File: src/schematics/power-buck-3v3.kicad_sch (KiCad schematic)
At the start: 12 parts, among them U14 INA219xxDCN, U4 TPS562202DRLR

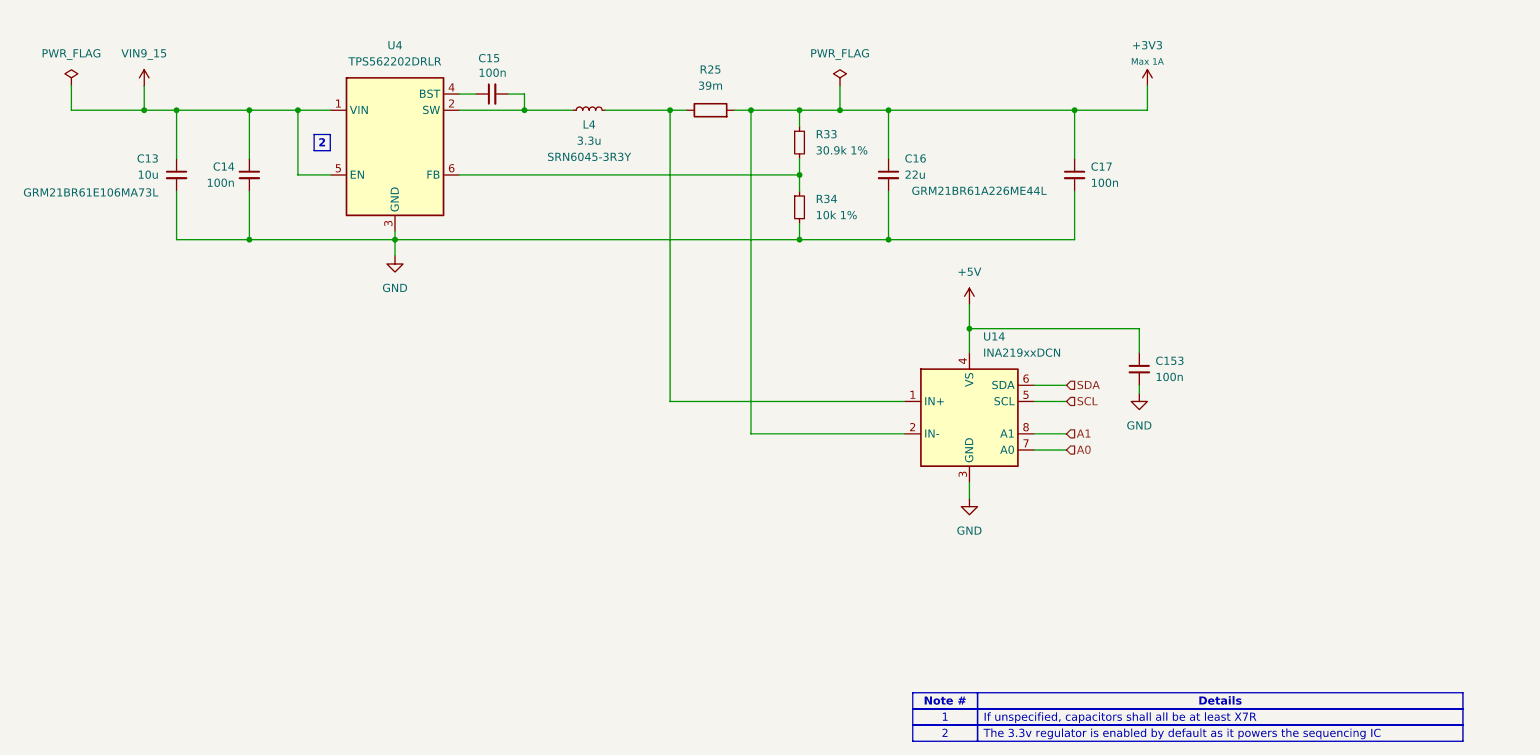
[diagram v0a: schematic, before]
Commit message: Add bom components
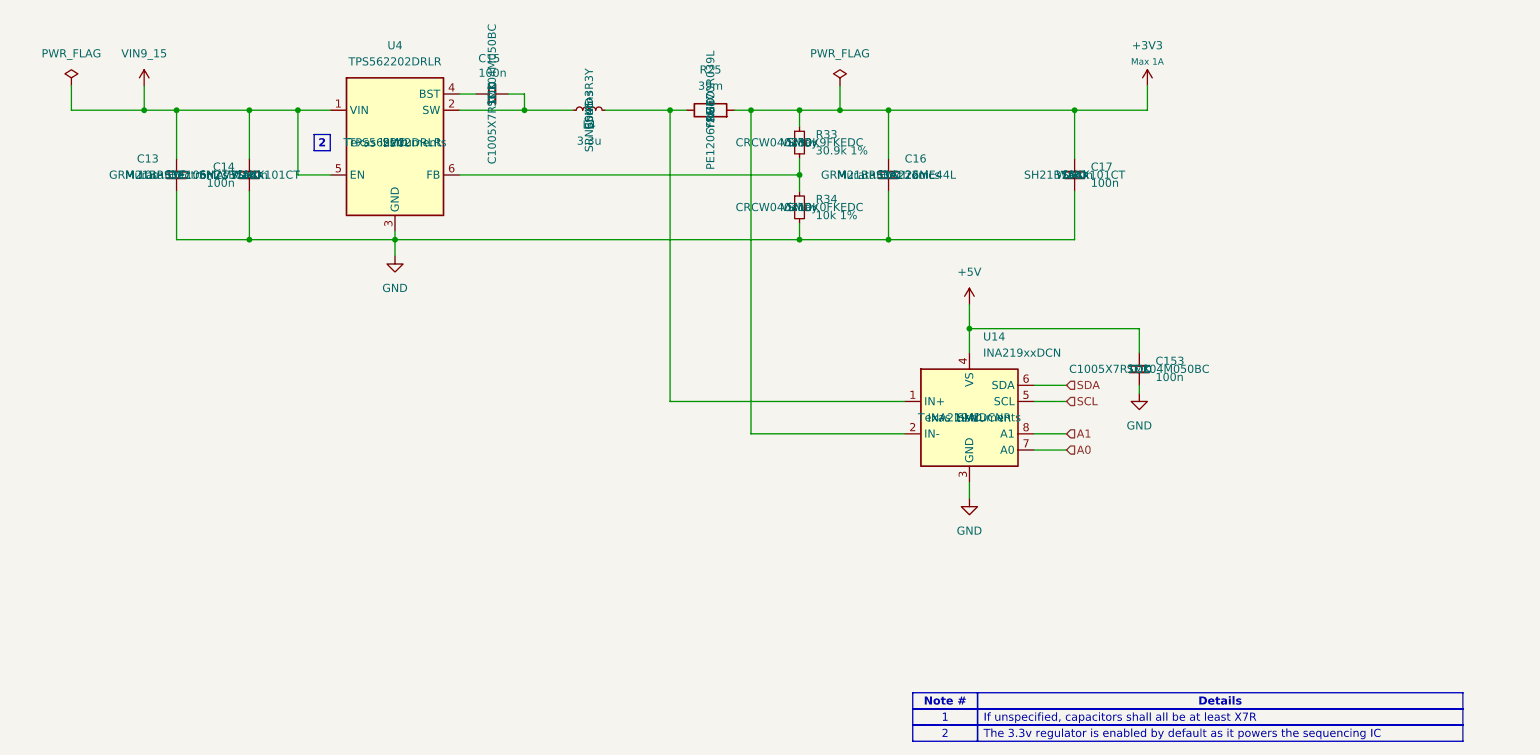
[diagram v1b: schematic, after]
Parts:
- C13: MPN (none) -> GRM21BR61E106MA73L; Manufacturer (none) -> Murata Electronics; Mouting Technology (none) -> SMD; Part GRM21BR61E106MA73L -> (none)
- C14, C17: MPN (none) -> SH21B104K101CT; Manufacturer (none) -> Walsin; Mouting Technology (none) -> SMD
- C15, C153: MPN (none) -> C1005X7R1C104M050BC; Manufacturer (none) -> TDK; Mouting Technology (none) -> SMD
- C16: MPN (none) -> GRM21BR61A226ME44L; Manufacturer (none) -> Murata Electronics; Mouting Technology (none) -> SMD; Part GRM21BR61A226ME44L -> (none)
- L4: MPN (none) -> SRN6045-3R3Y; Manufacturer (none) -> Bourns; Mouting Technology (none) -> SMD; Part SRN6045-3R3Y -> (none)
- R25: MPN (none) -> PE1206FRE470R039L; Manufacturer (none) -> YAGEO; Mouting Technology (none) -> SMD
- R33: MPN (none) -> CRCW040230K9FKEDC; Manufacturer (none) -> Vishay; Mouting Technology (none) -> SMD
- R34: MPN (none) -> CRCW040210K0FKEDC; Manufacturer (none) -> Vishay; Mouting Technology (none) -> SMD
- U14: MPN (none) -> INA219AIDCNR; Manufacturer (none) -> Texas Instruments; Mouting Technology (none) -> SMD
- U4: MPN (none) -> TPS562202DRLR; Manufacturer (none) -> Texas Instruments; Mouting Technology (none) -> SMD
